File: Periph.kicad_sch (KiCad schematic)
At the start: 11 parts, among them U10 ICM-42688-P, U9 W25Q128JVS

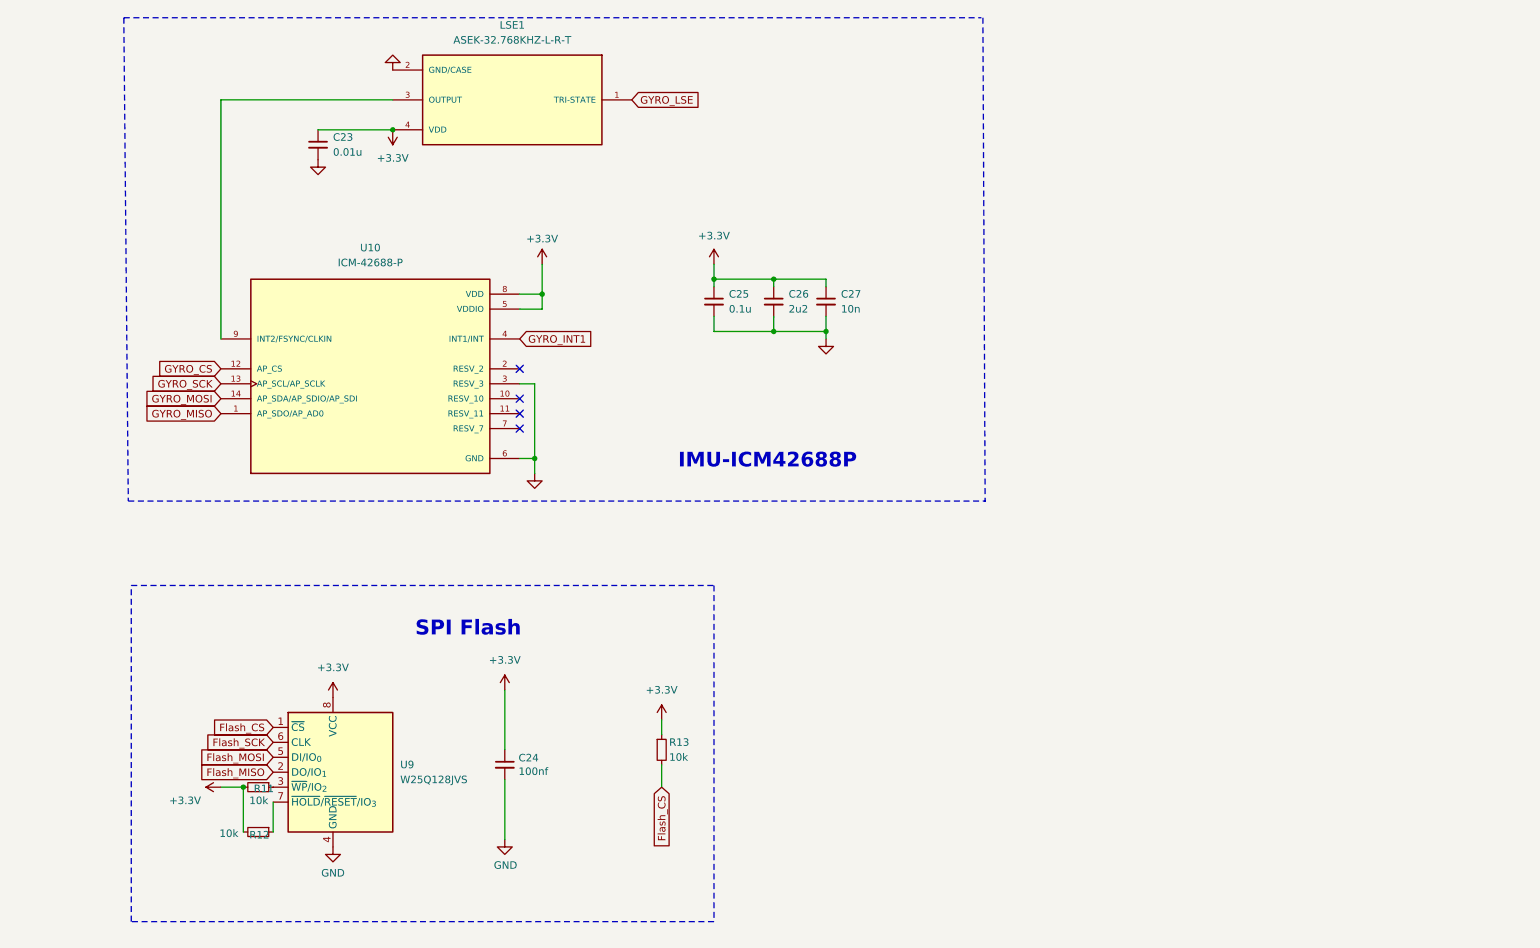
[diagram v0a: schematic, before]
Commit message: update
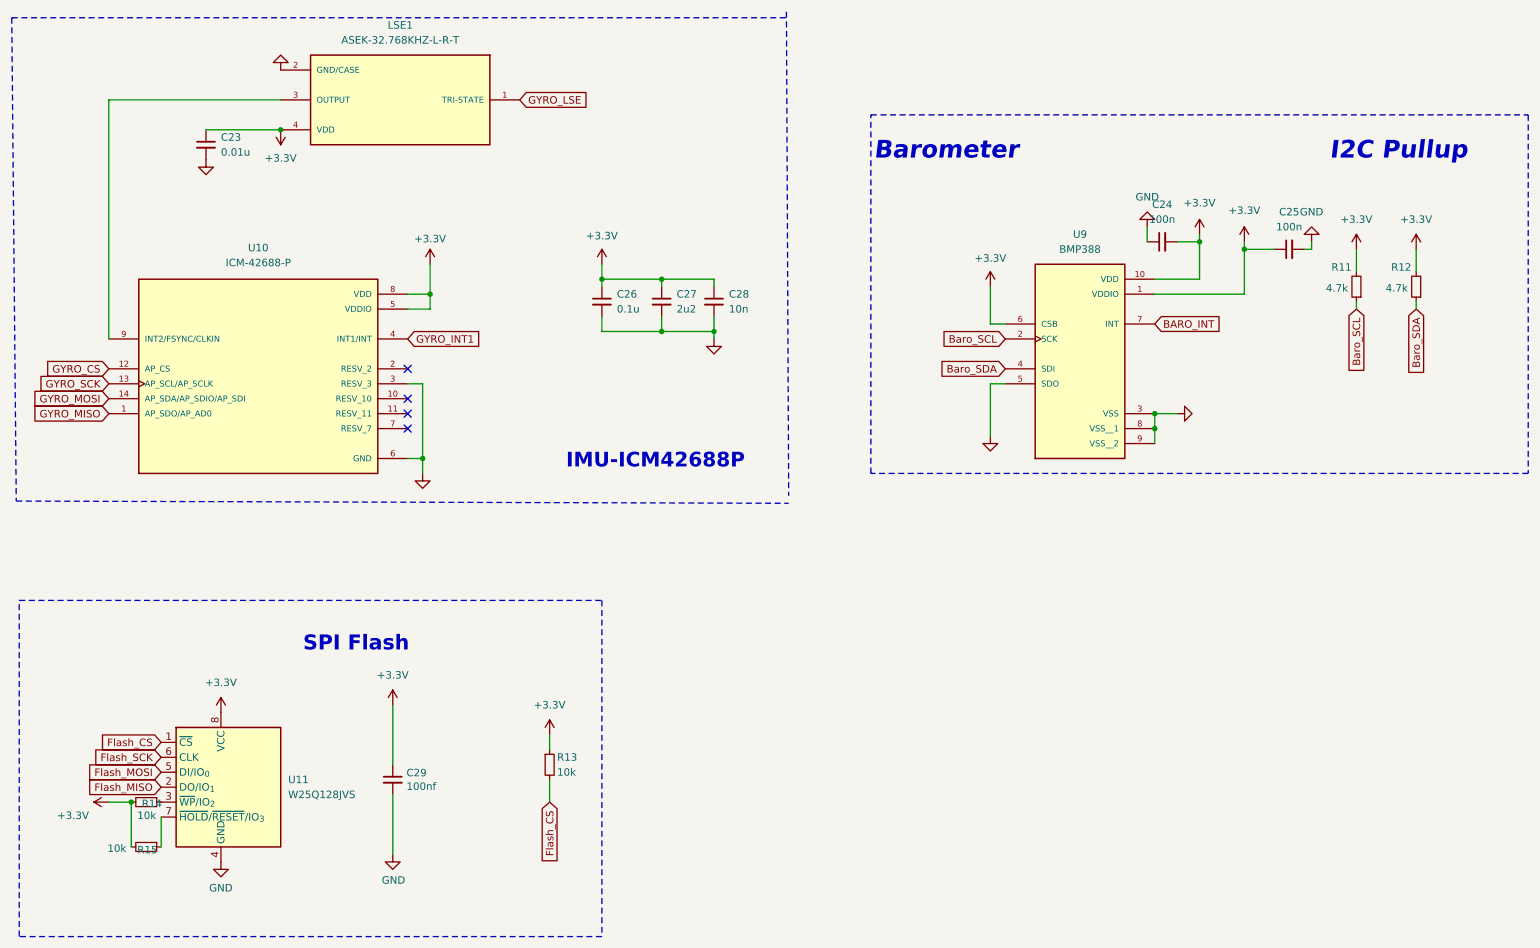
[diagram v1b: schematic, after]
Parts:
- added C24, C25: 100n, Capacitor_SMD:C_0201_0603Metric, symbol Device:C_Small
- added R11, R12: 4.7k, Resistor_SMD:R_0603_1608Metric, symbol Device:R_Small
- added U9: BMP388, mylib:BMP388, symbol BMP388:BMP388
- renumbered C25 to C26, C26 to C27, C27 to C28, C24 to C29, R11 to R14, R12 to R15, U9 to U11
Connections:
- net +3.3V: now also C24.2, C25.1, R11.2, R12.2, U9.1 (VDDIO), U9.10 (VDD), U9.6 (CSB)
- net GND: now also C24.1, C25.2, U9.3 (VSS), U9.5 (SDO), U9.8 (VSS__1), U9.9 (VSS__2)
- new net BARO_INT: U9.7 (INT)
- new net Baro_SCL: R11.1, U9.2 (SCK)
- new net Baro_SDA: R12.1, U9.4 (SDI)
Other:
- note added: "Barometer"
- note added: "I2C Pullup"
- moved on the sheet: C23, C26, C27, C28, C29, LSE1, R13, R14, R15, U10, U11
